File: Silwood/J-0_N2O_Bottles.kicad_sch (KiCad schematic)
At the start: 19 parts

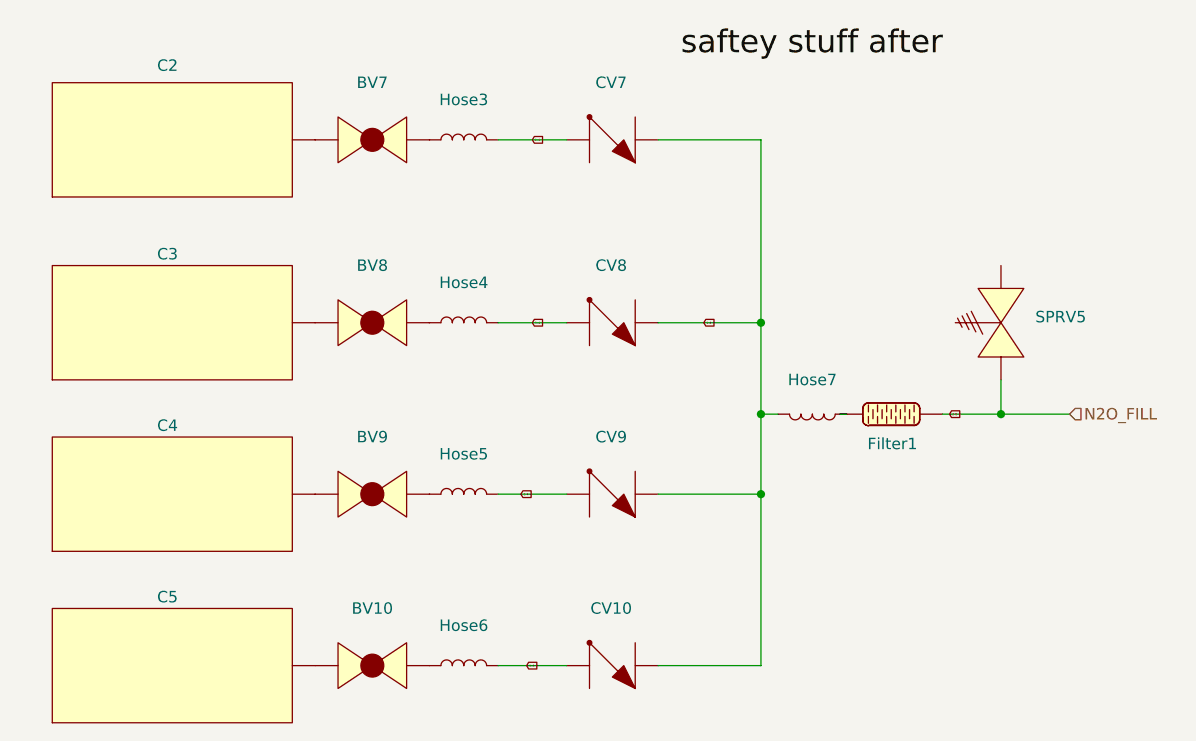
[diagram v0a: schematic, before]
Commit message: silwood upgrade
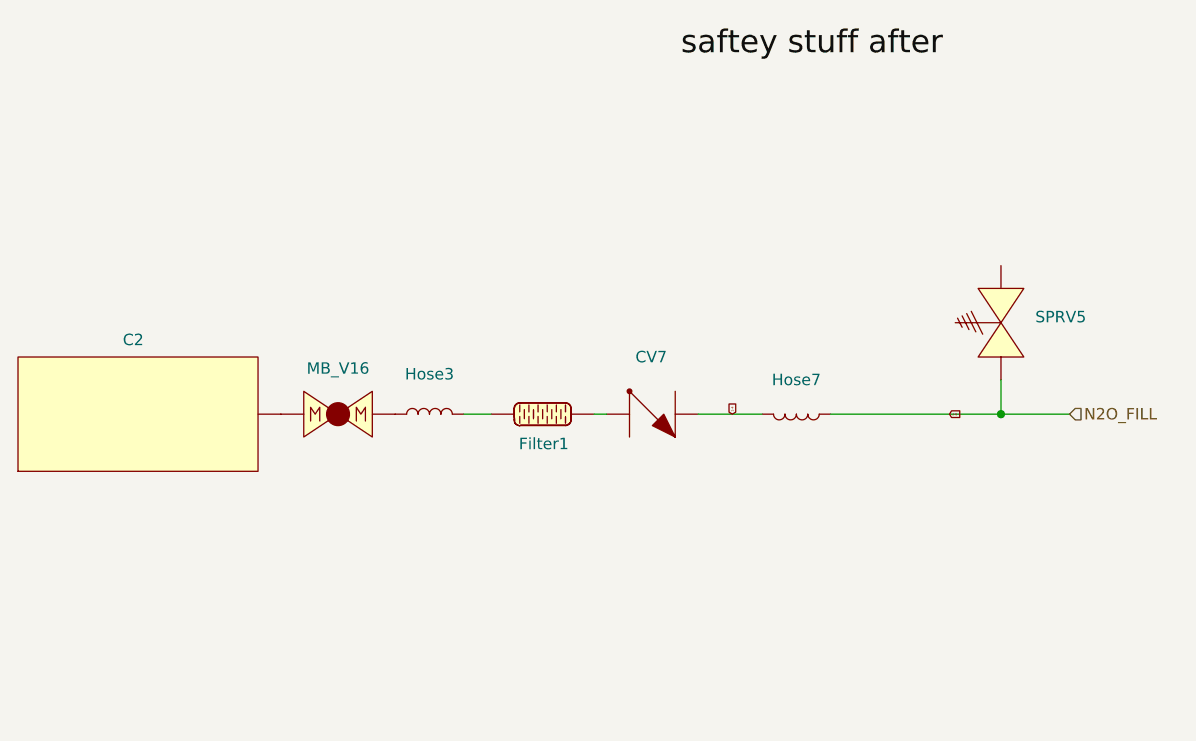
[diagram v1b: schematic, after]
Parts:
- removed BV10, BV7, BV8, BV9: ~, symbol PID_symbols:Ball_Valve
- removed C3, C4, C5: ~, symbol PID_symbols:Cylinder
- removed CV10, CV8, CV9: ~, symbol PID_symbols:Check_Valve
- removed Hose4, Hose5, Hose6: ~, symbol PID_symbols:Hose
- added MB_V16: ~, symbol PID_symbols:MBallValve
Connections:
- net 1-4: no longer Hose3.
- net 3-8: now also Hose7.; no longer Filter1.
- net at Hose3.: now also MB_V16.
- net at C2.: now also MB_V16.
- net at Filter1.: now also CV7.; no longer Hose7.
- new net: Filter1., Hose3.
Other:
- moved on the sheet: C2, CV7, Filter1, Hose3, Hose7
